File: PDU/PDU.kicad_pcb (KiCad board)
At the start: 2 copper layers, 111 x 127 mm, 82 parts, among them J10 Conn_01x02_Socket, J11 Screw_Terminal_01x02, J12 Conn_01x05_Pin, J2 USB_B_Micro, J3 Screw_Terminal_01x02, J4 Conn_01x03_Socket, J5 Conn_01x02_Socket, J6 Conn_01x02_Socket, J7 Conn_01x02_Socket, J8 Conn_01x02_Socket, J9 Conn_01x02_Socket, Q1 PMOS, Q2 NMOS, Q3 PMOS, U1 TPS564257DRLR, U2 MCP6002-I/P, U5 LM73100RPWR, U6 BQ25172DSGR, U8 MAX20801TPBA+, U9 TPS564257DRLR

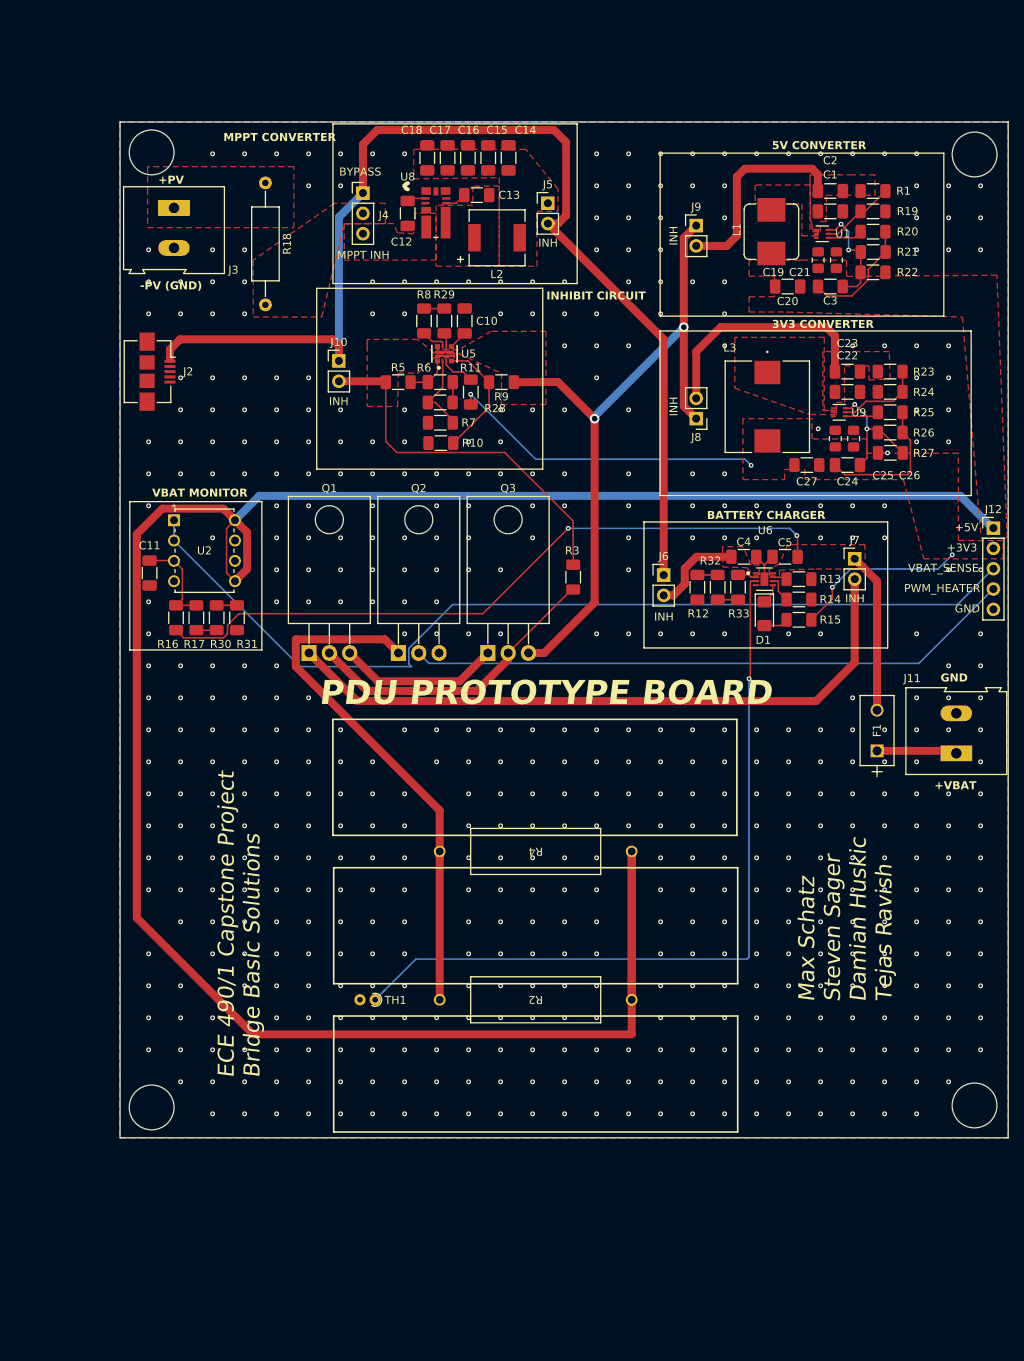
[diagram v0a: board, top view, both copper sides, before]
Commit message: Last revision
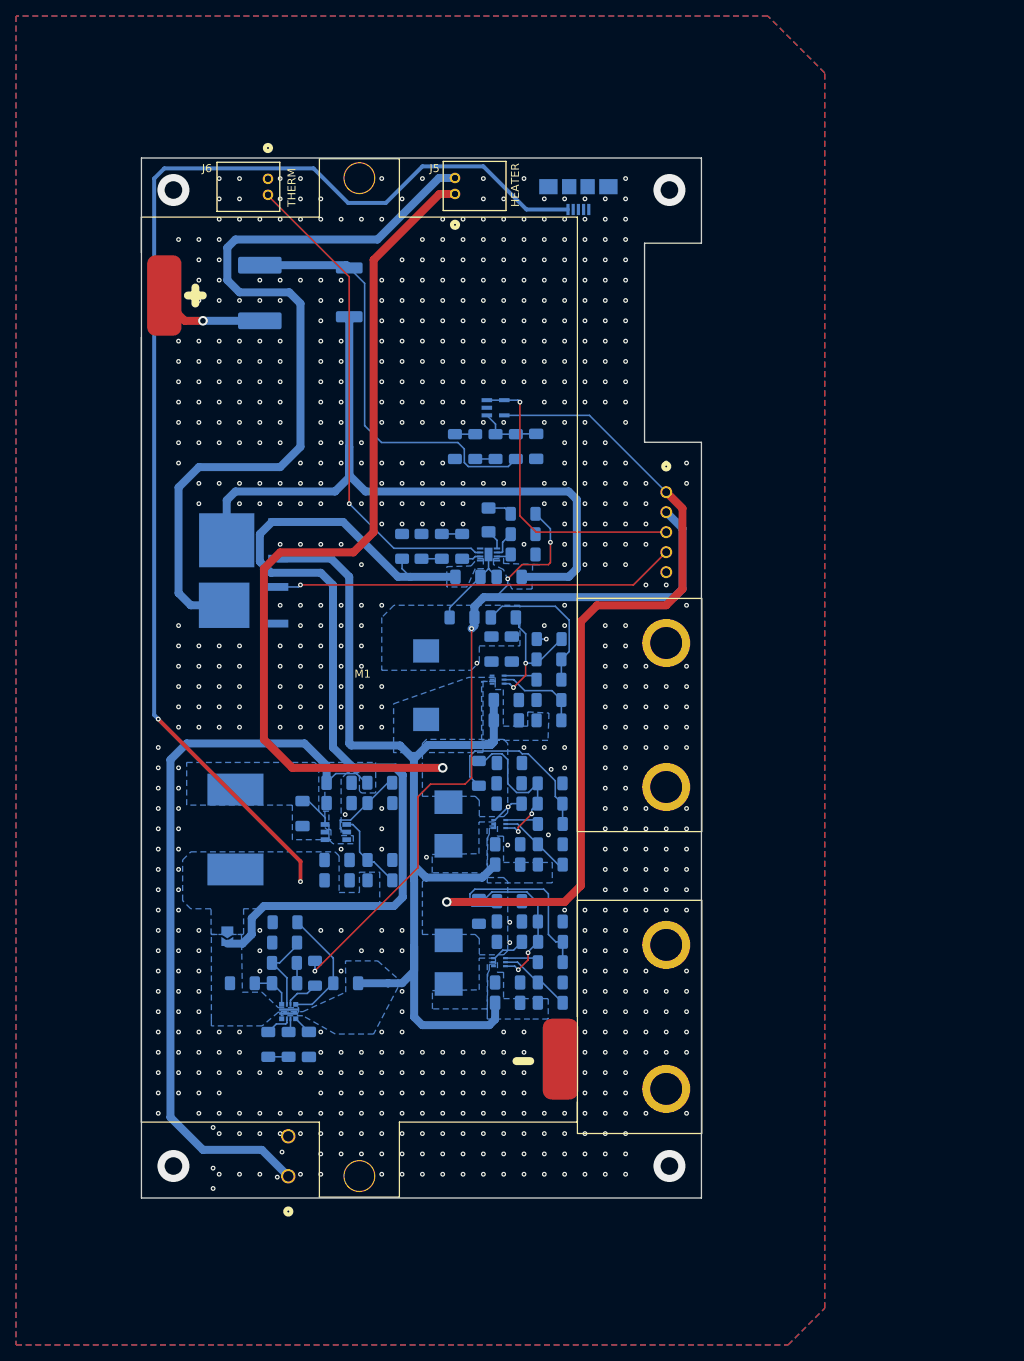
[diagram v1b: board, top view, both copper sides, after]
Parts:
- removed C12: 1u, Capacitor_SMD:C_1206_3216Metric_Pad1.33x1.80mm_HandSolder
- removed C13: 0.22u, Capacitor_SMD:C_1206_3216Metric_Pad1.33x1.80mm_HandSolder
- removed C14, C15, C16, C17, C18: 10u, Capacitor_SMD:C_1206_3216Metric_Pad1.33x1.80mm_HandSolder
- removed J10, J7, J8, J9: Conn_01x02_Socket, Connector_PinHeader_2.54mm:PinHeader_1x02_P2.54mm_Vertical
- removed J11: Screw_Terminal_01x02, TerminalBlock:TerminalBlock_Altech_AK300-2_P5.00mm
- removed J12: Conn_01x05_Pin, Connector_PinHeader_2.54mm:PinHeader_1x05_P2.54mm_Vertical
- removed J4: Conn_01x03_Socket, Connector_PinHeader_2.54mm:PinHeader_1x03_P2.54mm_Vertical
- removed L2: 0.68uH, Capstone:IND_RR68M8A_VIS
- removed Q1: PMOS, Package_TO_SOT_THT:TO-220-3_Horizontal_TabDown
- removed Q2: NMOS, Package_TO_SOT_THT:TO-220-3_Horizontal_TabDown
- removed R2, R4: 15, Capstone:res2_1-1625892-1_TEC
- removed TH1: 10k, Resistor_THT:R_Axial_DIN0204_L3.6mm_D1.6mm_P1.90mm_Vertical
- removed U8: MAX20801TPBA+, Capstone:21-100119_MXM
- added C28: 22u, Capacitor_SMD:C_1206_3216Metric_Pad1.33x1.80mm_HandSolder, B.Cu at (145.5, 111.7)
- added C29: 100n, Capacitor_SMD:C_1206_3216Metric_Pad1.33x1.80mm_HandSolder, B.Cu at (145.5, 109.1)
- added C30: 4.7u, Capacitor_SMD:C_1206_3216Metric_Pad1.33x1.80mm_HandSolder, B.Cu at (124.2, 114.1)
- added C31: 100n, Capacitor_SMD:C_1206_3216Metric_Pad1.33x1.80mm_HandSolder, B.Cu at (124.2, 111.6)
- added C32: 100n, Capacitor_SMD:C_1206_3216Metric_Pad1.33x1.80mm_HandSolder, B.Cu at (119.6, 115.4)
- added C33: 22u, Capacitor_SMD:C_1206_3216Metric_Pad1.33x1.80mm_HandSolder, B.Cu at (124.0, 121.2)
- added C34: 22u, Capacitor_SMD:C_1206_3216Metric_Pad1.33x1.80mm_HandSolder, B.Cu at (124.0, 123.8)
- added C6: 10u, Capacitor_SMD:C_1206_3216Metric_Pad1.33x1.80mm_HandSolder, B.Cu at (145.3, 121.8)
- added C7: 100n, Capacitor_SMD:C_1206_3216Metric_Pad1.33x1.80mm_HandSolder, B.Cu at (145.3, 119.3)
- added C8: 10p, Resistor_SMD:R_1206_3216Metric_Pad1.30x1.75mm_HandSolder, B.Cu at (141.7, 110.4)
- added C9: 22u, Capacitor_SMD:C_1206_3216Metric_Pad1.33x1.80mm_HandSolder, B.Cu at (145.5, 114.2)
- added H1: ReedSW MT, Capstone:ReedSW, F.Cu at (161.9, 103.1)
- added H2: ReedSW MT, Capstone:ReedSW, F.Cu at (161.9, 140.9)
- added J1: S5B-PH-K-S, Capstone:CONN_B5B-XH-A_JST, B.Cu at (165.1, 75.3)
- added JP1: SolderJumper_2_Open, Jumper:SolderJumper-2_P1.3mm_Open_TrianglePad1.0x1.5mm, B.Cu at (110.2, 130.8)
- added L4: 4.7u, Inductor_SMD:L_Bourns_SRP7028A_7.3x6.6mm, B.Cu at (137.9, 116.7)
- added L5: 15uH, Capstone:IND_BOURNS_SRR1208, B.Cu at (111.3, 117.4)
- added M1: ~, Capstone:AA_Bat_Contact, F.Cu at (126.7, 98.4)
- added MOSFET1: DMP10H400SK3-13, Capstone:TO252-DPAK-DMP10H400SK3_DIO, B.Cu at (110.2, 81.3)
- added R34: 113k, Resistor_SMD:R_1206_3216Metric_Pad1.30x1.75mm_HandSolder, B.Cu at (150.6, 121.8)
- added R35: 30k, Resistor_SMD:R_1206_3216Metric_Pad1.30x1.75mm_HandSolder, B.Cu at (150.6, 119.3)
- added R36: 10k, Resistor_SMD:R_1206_3216Metric_Pad1.30x1.75mm_HandSolder, B.Cu at (150.6, 116.7)
- added R37: 75.2k, Resistor_SMD:R_1206_3216Metric_Pad1.30x1.75mm_HandSolder, B.Cu at (150.6, 114.2)
- added R38: 10k, Resistor_SMD:R_1206_3216Metric_Pad1.30x1.75mm_HandSolder, B.Cu at (150.6, 111.7)
- added R40: 100k, Resistor_SMD:R_1206_3216Metric_Pad1.30x1.75mm_HandSolder, B.Cu at (132.1, 82.0)
- added R41: 7.15k, Resistor_SMD:R_1206_3216Metric_Pad1.30x1.75mm_HandSolder, B.Cu at (129.3, 121.2)
- added R42: Rent, Resistor_SMD:R_1206_3216Metric_Pad1.30x1.75mm_HandSolder, B.Cu at (129.3, 111.6)
- added R43: Renb, Resistor_SMD:R_1206_3216Metric_Pad1.30x1.75mm_HandSolder, B.Cu at (129.3, 114.1)
- added U3: TPS564257DRLR, Capstone:TPS564242DRLR_TEX, B.Cu at (144.3, 116.8)
- added U4: MCP6001UT-I/OT, Capstone:SOT-23-5_MC_MCH, B.Cu at (143.8, 64.7)
- C1, C10, C11, C2, C20, C22, C23, C24, C27, C3, C4, C5, D1, J2, L1, L3, R10, R11, R12, R13, R14, R15, R16, R17, R19, R20, R22, R23, R24, R25, R26, R27, R28, R29, R30, R31, R32, R33, R5, R6, R7, R8, R9, U1, U5, U6, U9: moved to B.Cu
- C19, C21, C25, C26: footprint Capacitor_SMD:C_0805_2012Metric_Pad1.18x1.45mm_HandSolder -> Capacitor_SMD:C_1206_3216Metric_Pad1.33x1.80mm_HandSolder; moved to B.Cu
- F1: footprint Capstone:FUS_LITTELFUSE_392_LTF -> Fuse:Fuse_2920_7451Metric_Pad2.10x5.45mm_HandSolder; moved to B.Cu
- J3: value Screw_Terminal_01x02 -> 1935310; footprint TerminalBlock:TerminalBlock_Altech_AK300-2_P5.00mm -> Capstone:CONN_1935310_PXC; moved to B.Cu
- J5, J6: value Conn_01x02_Socket -> S2B-PH-K-SLFSN; footprint Connector_PinHeader_2.54mm:PinHeader_1x02_P2.54mm_Vertical -> Capstone:CONN_S2B-PH-K-S_JST
- Q3: value PMOS -> IPD60R2K0PFD7SAUMA1; footprint Package_TO_SOT_THT:TO-220-3_Horizontal_TabDown -> Capstone:DPAK229P994X240-3N; moved to B.Cu
- R1: value 137k -> 113k; moved to B.Cu
- R18: value R -> 100k; footprint Resistor_THT:R_Axial_DIN0309_L9.0mm_D3.2mm_P15.24mm_Horizontal -> Resistor_SMD:R_1206_3216Metric_Pad1.30x1.75mm_HandSolder; moved to B.Cu
- R21: value 220k -> 75.2k; moved to B.Cu
- R3: value 10k -> 10; footprint Resistor_SMD:R_1206_3216Metric_Pad1.30x1.75mm_HandSolder -> Resistor_SMD:R_2512_6332Metric_Pad1.40x3.35mm_HandSolder; moved to B.Cu
- U2: value MCP6002-I/P -> LMR51625XFDDCR; footprint Capstone:PDIP8_300MC_MCH -> Capstone:DDC0006A-MFG; moved to B.Cu
- moved J3 121.9 mm to (117.9, 160.8), turned to 90 degrees
- moved C2 109.2 mm to (145.3, 139.1)
- moved R1 109.2 mm to (150.6, 139.1)
- moved C1 104.5 mm to (145.3, 136.6)
- moved R19 104.5 mm to (150.6, 136.6)
- moved L1 99.8 mm to (137.9, 134.0), turned to 90 degrees
- moved R20 99.8 mm to (150.6, 134.0)
- moved U1 99.6 mm to (144.3, 134.0)
- moved F1 96.1 mm to (114.3, 50.4)
- moved R21 95.2 mm to (150.6, 131.5)
- moved C21 94.5 mm to (145.5, 131.5), turned to 0 degrees
- moved C10 92.5 mm to (120.4, 144.3), turned to -90 degrees
- moved R29 92.5 mm to (117.9, 144.3), turned to 90 degrees
- moved R8 92.5 mm to (115.4, 144.3), turned to -90 degrees
- moved R22 90.6 mm to (150.6, 128.9)
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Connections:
- C1 pad 1: Net-(J9-Pin_2) -> /Converters/VIN
- C2 pad 1: Net-(J9-Pin_2) -> /Converters/VIN
- C22 pad 1: Net-(J8-Pin_2) -> /Converters/VIN
- C23 pad 1: Net-(J8-Pin_2) -> /Converters/VIN
- C4 pad 1: /NiMH Charger/IN -> /Ideal Diode/IN
- F1 pad 2: /NiMH Charger/OUT -> /VBAT_Monitor/VBAT_IN
- J2 pad 1: /MPPT/MPPT_OUT -> /MPPT/+12V
- J3 pad 1: Net-(J3-Pin_1) -> /MPPT/VIN
- J5 pad 1: Net-(J5-Pin_1) -> +5V_HEATER
- J5 pad 2: /MPPT/MPPT_OUT -> Net-(J5-Pad2)
- J6 pad 1: /MPPT/MPPT_OUT -> GND
- J6 pad 2: /NiMH Charger/IN -> Net-(U6-TS)
- Q3 pad 1: Net-(Q1-S) -> /PWM_HEATER
- Q3 pad 3: /Converters/VIN -> GND
- R1 pad 1: Net-(J9-Pin_2) -> /Converters/VIN
- R16 pad 1: /NiMH Charger/OUT -> /VBAT_Monitor/VBAT_IN
- R18 pad 1: Net-(J3-Pin_1) -> /MPPT/+12V
- R18 pad 2: Net-(J4-Pin_2) -> Net-(U2-FB)
- R23 pad 1: Net-(J8-Pin_2) -> /Converters/VIN
- R3 pad 1: /Ideal Diode/IN -> /NiMH Charger/OUT
- R3 pad 2: Net-(Q1-G) -> /VBAT_Monitor/VBAT_IN
- U1 pad 1: Net-(J9-Pin_2) -> /Converters/VIN
- U2 pad 1: /VBAT_SENSE -> Net-(U2-FB)
- U2 pad 2: /VBAT_SENSE -> Net-(U2-EN)
- U2 pad 3: /VBAT_Monitor/VINA+ -> /MPPT/VIN
- U2 pad 5: +5V -> Net-(U2-SW)
- U2 pad 6: GND -> Net-(U2-CB)
- U6 pad 1: /NiMH Charger/IN -> /Ideal Diode/IN
- U9 pad 1: Net-(J8-Pin_2) -> /Converters/VIN
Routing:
- net +5V: track 301.0 -> 127.3 mm, vias 0 -> 1
- net /MPPT/+12V: track 0.00 -> 153.6 mm, vias 0 -> 2
- net /MPPT/MPPT_OUT: track 142.0 -> 0.00 mm
- net +5V_HEATER: track 0.00 -> 130.8 mm, vias 0 -> 1
- net Net-(J5-Pad2): track 0.00 -> 101.3 mm
- net /MPPT/VIN: track 0.00 -> 92.2 mm
- net Net-(J7-Pin_2): track 83.1 -> 0.00 mm
- net /VBAT_SENSE: track 118.3 -> 37.6 mm, vias 0 -> 1
- net /Ideal Diode/IN: track 46.3 -> 115.8 mm
- net Net-(Q2-D): track 66.0 -> 0.00 mm
- net /VBAT_Monitor/VBAT_IN: track 0.00 -> 54.2 mm
- net +3.3V: track 79.8 -> 131.7 mm
- net Net-(Q1-G): track 38.2 -> 0.00 mm
- net /Converters/VIN: track 87.3 -> 123.0 mm, vias 2 -> 0
- net Net-(U6-TS): track 97.0 -> 61.6 mm
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- added copper zone on B.Cu, net +3.3V
- added copper zone on B.Cu, net +5V
- added copper zone on B.Cu, net +5V_HEATER
- added copper zone on B.Cu, net /Converters/VIN
- added copper zone on B.Cu, net /Ideal Diode/IN
- added copper zone on B.Cu, net /MPPT/+12V
- added copper zone on B.Cu, net /MPPT/VIN
- added copper zone on B.Cu, net /NiMH Charger/OUT
- added copper zone on B.Cu, net Net-(U1-SW)
- added copper zone on B.Cu, net Net-(U2-SW)
- added copper zone on B.Cu, net Net-(U3-SW)
- added copper zone on B.Cu, net Net-(U9-SW)
- removed copper zone on F.Cu, net +3.3V
- removed copper zone on F.Cu, net +5V
- removed copper zone on F.Cu, net /Converters/VIN
- removed copper zone on F.Cu, net /Ideal Diode/IN
- removed copper zone on F.Cu, net /MPPT/PV+
- removed copper zone on F.Cu, net /NiMH Charger/IN
- removed copper zone on F.Cu, net /NiMH Charger/OUT
- removed copper zone on F.Cu, net Net-(J3-Pin_1)
- removed copper zone on F.Cu, net Net-(J4-Pin_2)
- removed copper zone on F.Cu, net Net-(J5-Pin_1)
- removed copper zone on F.Cu, net Net-(J8-Pin_2)
- removed copper zone on F.Cu, net Net-(J9-Pin_2)
- removed copper zone on F.Cu, net Net-(U1-SW)
- removed copper zone on F.Cu, net Net-(U8-OUT)
- removed copper zone on F.Cu, net Net-(U9-SW)
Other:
- board size 111 x 127 mm -> 70 x 130 mm
- board text added: "CHARGE"
- board text added: "ECE 490/1 CAPSTONE SSULPEP PDU BRIDGE BASIC SOLUTIONS"
- board text added: "HEATER"
- board text added: "PDU BOARD"
- board text added: "PV+"
- board text added: "PV-"
- board text added: "THERM"
- board text removed: "+PV"
- board text removed: "+VBAT"
- board text removed: "-PV (GND)"
- board text removed: "3V3 CONVERTER"
- board text removed: "5V CONVERTER"
- board text removed: "BATTERY CHARGER"
- board text removed: "BYPASS"
- board text removed: "ECE 490/1 Capstone Project Bridge Basic Solutions"
- board text removed: "INH"
- board text removed: "INHIBIT CIRCUIT"
- board text removed: "MPPT CONVERTER"
- board text removed: "MPPT INH"
- board text removed: "PDU PROTOTYPE BOARD"
- board text removed: "VBAT MONITOR"
